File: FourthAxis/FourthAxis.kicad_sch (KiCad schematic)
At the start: 1 part, among them U1 ESP32-WROOM-32

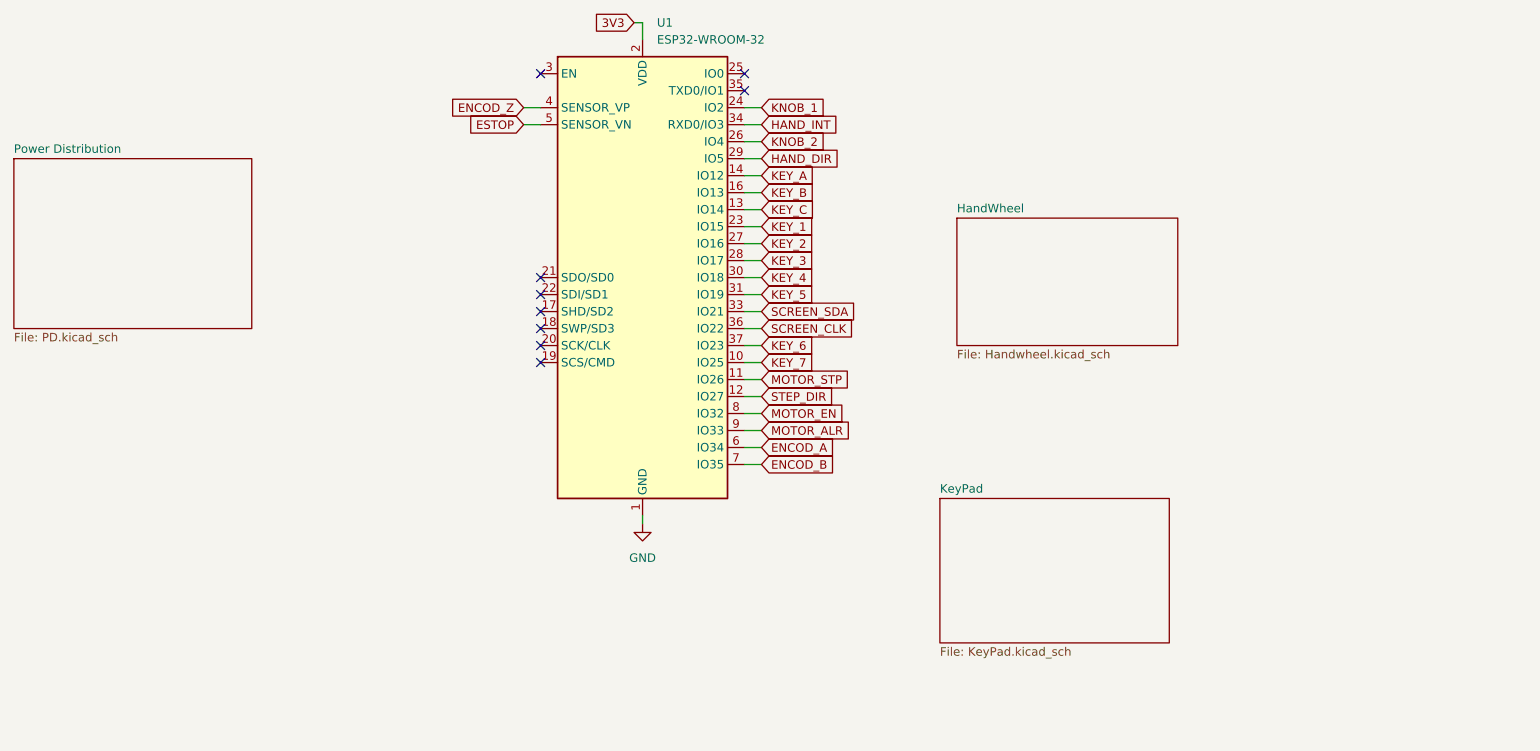
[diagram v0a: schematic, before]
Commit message: Keypad schem work
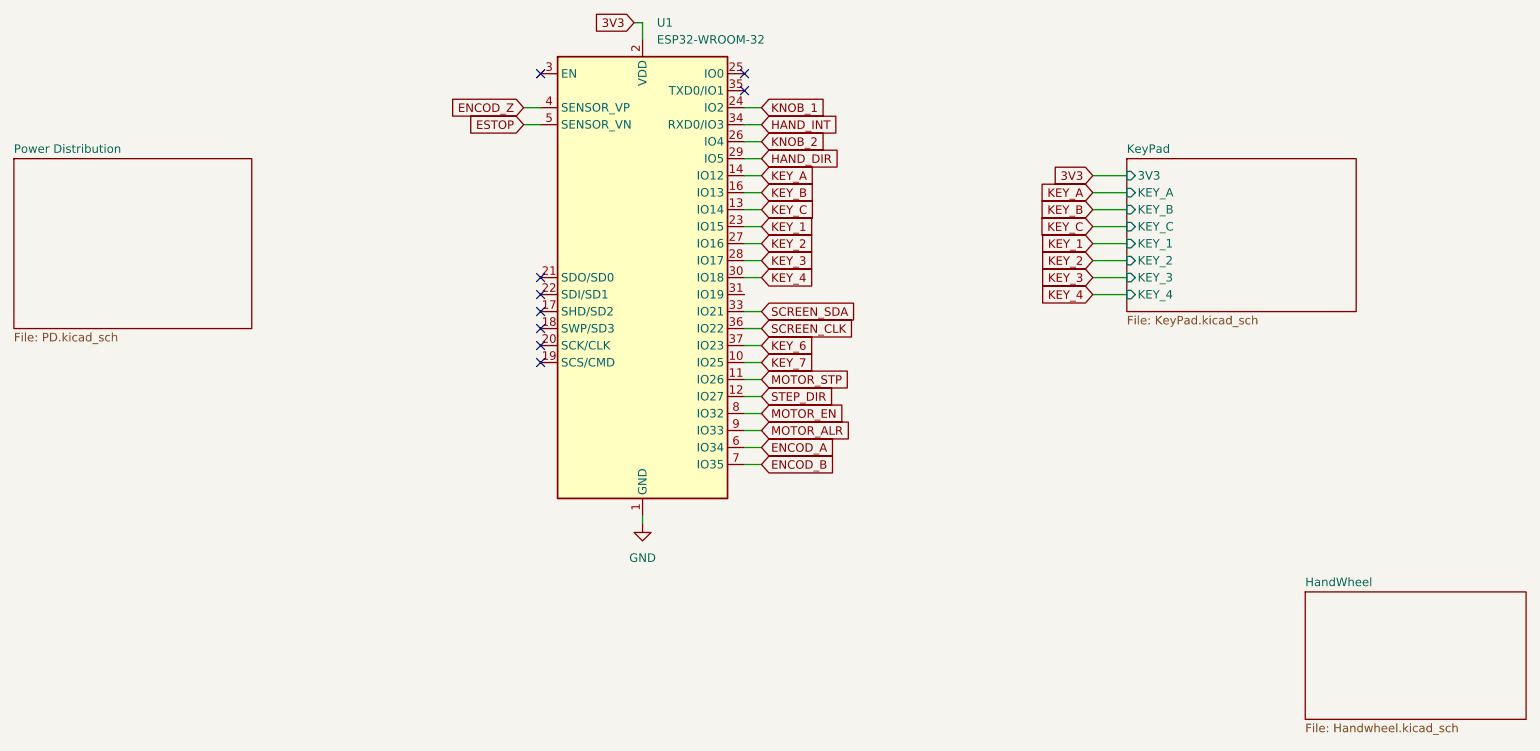
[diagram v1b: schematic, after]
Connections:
- net KEY_5: no longer names the net of U1.31 (IO19)
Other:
- sheet KeyPad ports: added 3V3, KEY_1, KEY_2, KEY_3, KEY_4, KEY_A, KEY_B, KEY_C; removed none
